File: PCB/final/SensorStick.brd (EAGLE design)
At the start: 74.9 x 39.4 mm, 56 parts, among them U1 TPD4F003DQDR, Y1 ECS-TXO-3225MV-400-TR

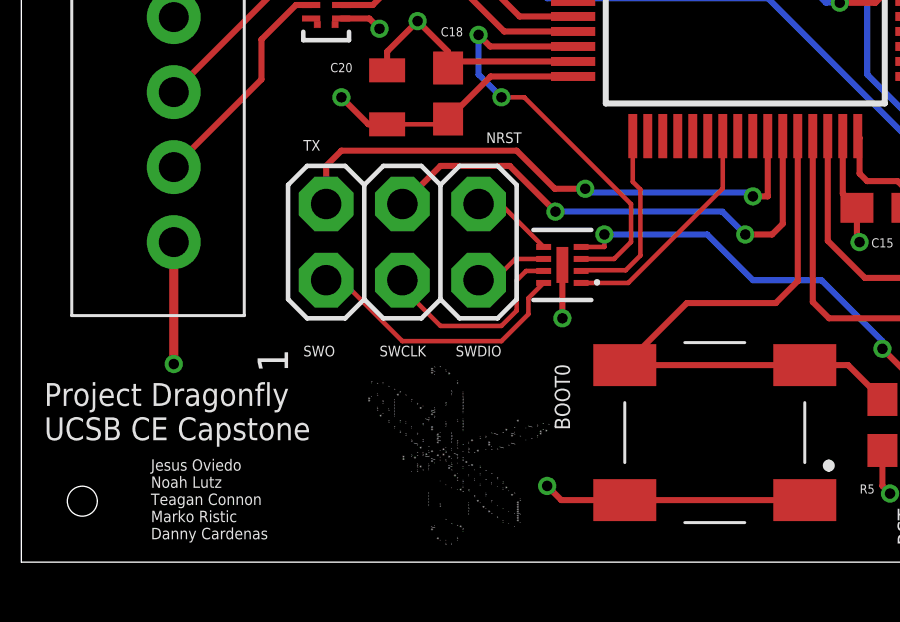
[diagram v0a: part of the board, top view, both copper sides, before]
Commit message: Jesus - Moved dfly to not cause probs
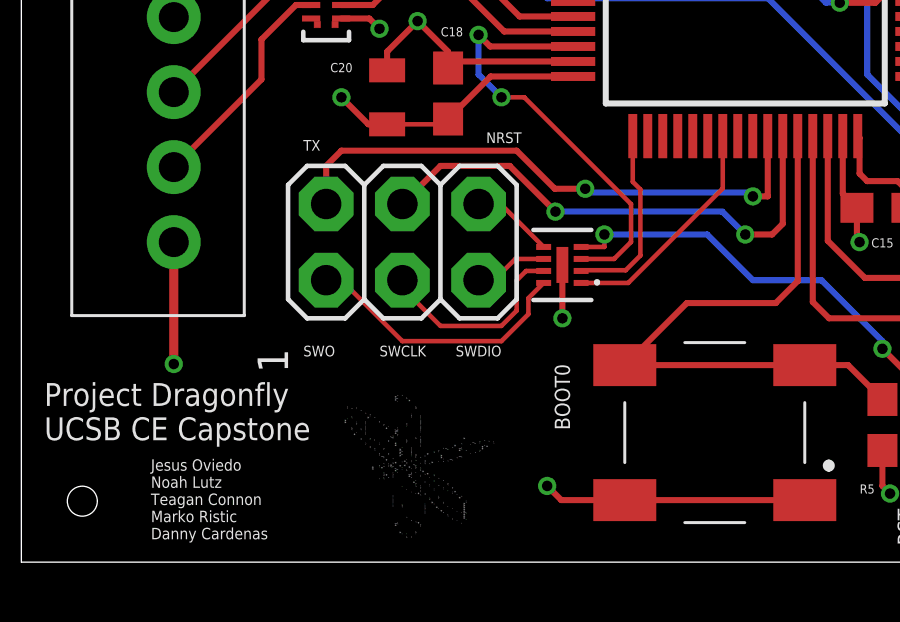
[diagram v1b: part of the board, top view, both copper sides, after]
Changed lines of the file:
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@@
 Danny Cardenas</text>
 <text x="50.8" y="22.606" size="1.016" layer="21" rot="R270">1</text>
-<text x="21.59" y="0.508" size="0.127" layer="21" rot="R90">
+<text x="18.796" y="0.762" size="0.1016" layer="21" rot="R90">
                                                                                                  **.        .,
                                                                                            ,,.       ,.      ,
@@
 <wire x1="68.326" y1="27.178" x2="65.786" y2="27.178" width="0.2032" layer="1"/>
 <via x="65.786" y="27.178" extent="1-16" drill="0.35"/>
-<wire x1="69.596" y1="18.796" x2="68.326" y2="27.178" width="0" layer="19" extent="1-1"/>
-<wire x1="65.278" y1="1.016" x2="67.056" y2="18.796" width="0" layer="19" extent="1-1"/>
-<wire x1="48.768" y1="26.162" x2="65.786" y2="27.178" width="0" layer="19" extent="1-1"/>
-<wire x1="37.951" y1="30.615" x2="45.72" y2="23.202" width="0" layer="19" extent="1-1"/>
-<wire x1="27.178" y1="29.464" x2="33.02" y2="32.584" width="0" layer="19" extent="1-1"/>
-<wire x1="22.733" y1="30.298" x2="27.178" y2="29.464" width="0" layer="19" extent="1-1"/>
-<wire x1="16.166" y1="31.171" x2="17.616" y2="31.821" width="0" layer="19" extent="1-1"/>
-<wire x1="15.24" y1="27.686" x2="14.224" y2="28.702" width="0" layer="19" extent="1-1"/>
-<wire x1="8.725" y1="28.763" x2="11.176" y2="30.3403" width="0" layer="19" extent="1-1"/>
-<wire x1="32.258" y1="24.5237" x2="26.88" y2="25.677" width="0" layer="19" extent="1-1"/>
-<wire x1="31.75" y1="17.272" x2="32.258" y2="24.5237" width="0" layer="19" extent="1-1"/>
-<wire x1="27.88" y1="14.201" x2="29.868" y2="16.189" width="0" layer="19" extent="1-1"/>
-<wire x1="31.584" y1="8.128" x2="30.734" y2="11.938" width="0" layer="19" extent="1-1"/>
-<wire x1="35.814" y1="10.16" x2="32.766" y2="8.2578" width="0" layer="19" extent="1-1"/>
-<wire x1="26.114" y1="2.068" x2="31.584" y2="8.128" width="0" layer="19" extent="1-1"/>
-<wire x1="8.382" y1="20.066" x2="4.318" y2="27.178" width="0" layer="19" extent="1-1"/>
-<wire x1="10.668" y1="15.494" x2="9.66" y2="19.471" width="0" layer="19" extent="1-1"/>
 </signal>
 <signal name="USART1_RX">
@@
 <wire x1="68.326" y1="29.718" x2="67.31" y2="29.718" width="0.2032" layer="1"/>
 <via x="67.31" y="29.718" extent="1-16" drill="0.35"/>
-<wire x1="49.739" y1="29.38" x2="67.31" y2="29.718" width="0" layer="19" extent="1-1"/>
-<wire x1="46.736" y1="29.376" x2="49.739" y2="29.38" width="0" layer="19" extent="1-1"/>
-<wire x1="40.281" y1="29.615" x2="40.281" y2="30.115" width="0" layer="19" extent="1-1"/>
-<wire x1="40.281" y1="31.115" x2="40.281" y2="30.115" width="0" layer="19" extent="1-1"/>
-<wire x1="33.02" y1="30.226" x2="40.281" y2="30.115" width="0" layer="19" extent="1-1"/>
-<wire x1="28.956" y1="29.464" x2="33.02" y2="30.226" width="0" layer="19" extent="1-1"/>
-<wire x1="29.868" y1="21.689" x2="27.38" y2="25.677" width="0" layer="19" extent="1-1"/>
-<wire x1="35.814" y1="17.526" x2="35.19" y2="21.336" width="0" layer="19" extent="1-1"/>
-<wire x1="32.004" y1="13.832" x2="36.764" y2="14.612" width="0" layer="19" extent="1-1"/>
-<wire x1="27.852" y1="11.811" x2="32.004" y2="12.7" width="0" layer="19" extent="1-1"/>
-<wire x1="20.88" y1="25.677" x2="27.38" y2="25.677" width="0" layer="19" extent="1-1"/>
-<wire x1="13.843" y1="27.504" x2="15.494" y2="28.956" width="0" layer="19" extent="1-1"/>
-<wire x1="10.16" y1="27.813" x2="11.595" y2="27.813" width="0" layer="19" extent="1-1"/>
-<wire x1="15.24" y1="24.384" x2="14.986" y2="26.576" width="0" layer="19" extent="1-1"/>
-<wire x1="13.208" y1="30.425" x2="15.494" y2="28.956" width="0" layer="19" extent="1-1"/>
-<wire x1="17.616" y1="32.471" x2="16.166" y2="31.821" width="0" layer="19" extent="1-1"/>
-<wire x1="12.446" y1="24.185" x2="15.24" y2="24.384" width="0" layer="19" extent="1-1"/>
-<wire x1="11.938" y1="21.082" x2="12.954" y2="22.098" width="0" layer="19" extent="1-1"/>
-<wire x1="10.66" y1="18.121" x2="10.66" y2="19.471" width="0" layer="19" extent="1-1"/>
-<wire x1="13.208" y1="18.034" x2="11.938" y2="17.78" width="0" layer="19" extent="1-1"/>
-<wire x1="18.034" y1="9.906" x2="18.392" y2="16.689" width="0" layer="19" extent="1-1"/>
-<wire x1="28.702" y1="3.722" x2="27.94" y2="10.668" width="0" layer="19" extent="1-1"/>
-<wire x1="29.718" y1="2.54" x2="28.956" y2="2.286" width="0" layer="19" extent="1-1"/>
-<wire x1="37.544" y1="1.56" x2="31.544" y2="1.56" width="0" layer="19" extent="1-1"/>
-<wire x1="40.386" y1="3.81" x2="39.624" y2="1.524" width="0" layer="19" extent="1-1"/>
-<wire x1="5.08" y1="10.668" x2="12.192" y2="16.394" width="0" layer="19" extent="1-1"/>
-<wire x1="68.326" y1="29.718" x2="67.31" y2="29.718" width="0" layer="19"/>
 </signal>
 <signal name="I2C2_SCL">
@@
 <wire x1="65.278" y1="37.338" x2="62.992" y2="35.052" width="0.2032" layer="1"/>
 <wire x1="62.738" y1="35.052" x2="62.992" y2="35.052" width="0.2032" layer="1"/>
-<wire x1="62.738" y1="35.052" x2="68.326" y2="37.338" width="0" layer="19"/>
 </signal>
 <signal name="GPIO_EXTI3">
